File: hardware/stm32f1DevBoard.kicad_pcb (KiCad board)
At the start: 2 copper layers, 105.4 x 62.2 mm, 67 parts, among them J1 USB_2, J2 POWER_JACK, J3 SDCARD, M1 Mounting Hole, M2 Mounting Hole, M3 Mounting Hole, M4 Mounting Hole, P1 JTAG, P2 P20, P3 P20, P4 WIFIDEBUG, Q1 MOSFET-P, U1 STM32F102C6, U2 MRF24WB0MX, U3 LM358, U4 VREG-X-5, U5 VREG-5-3.3, X1 32,768Hz, X2 20MHz

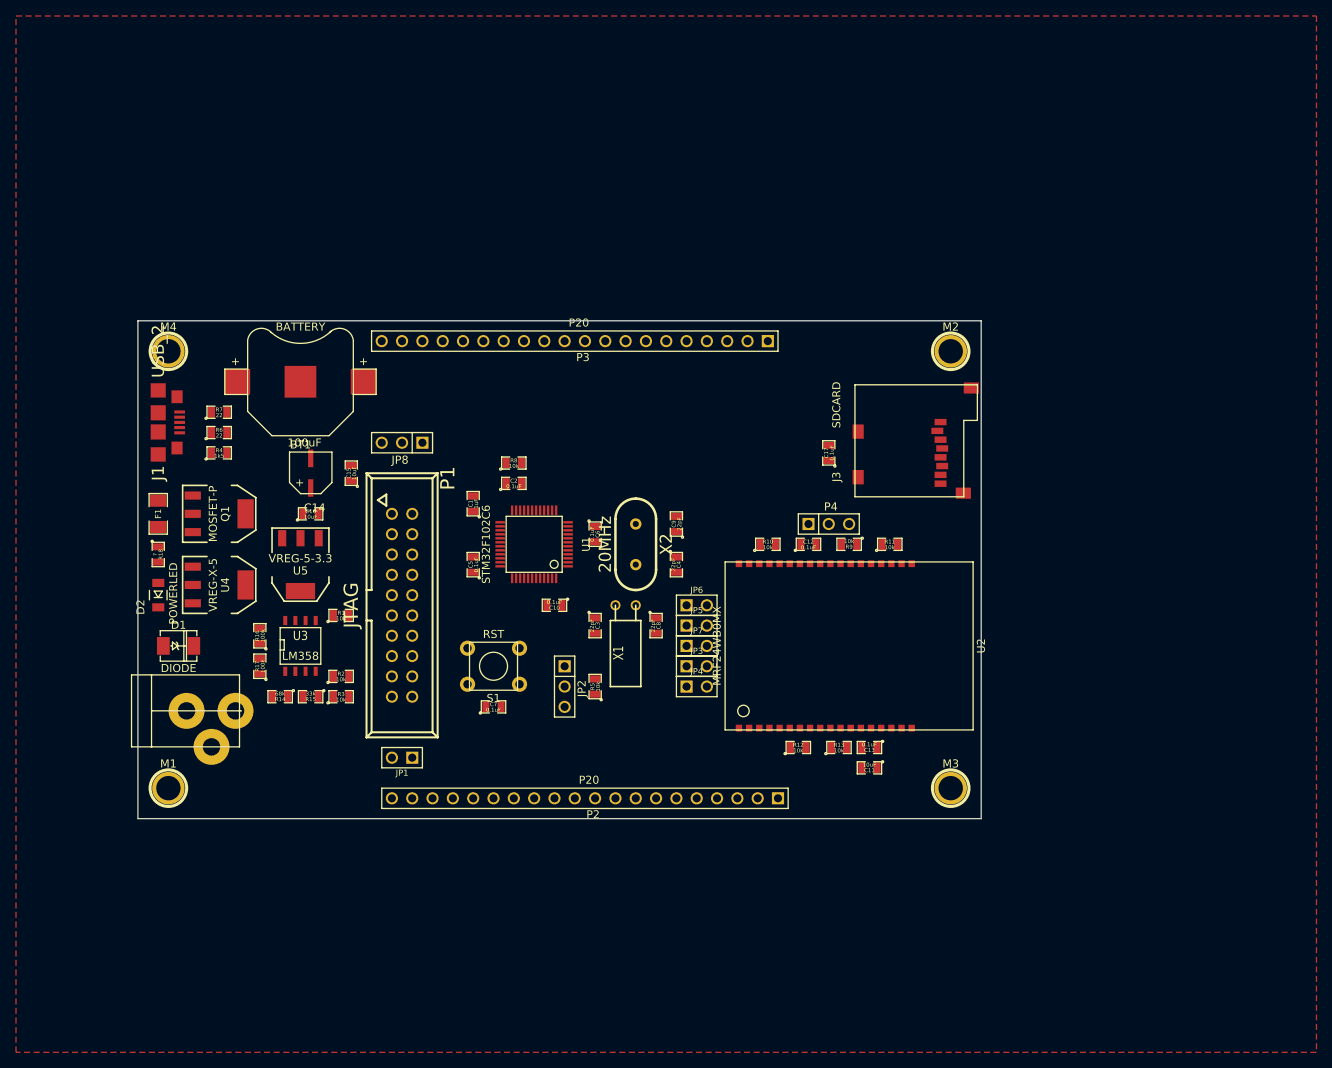
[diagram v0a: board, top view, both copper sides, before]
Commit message: layout complete
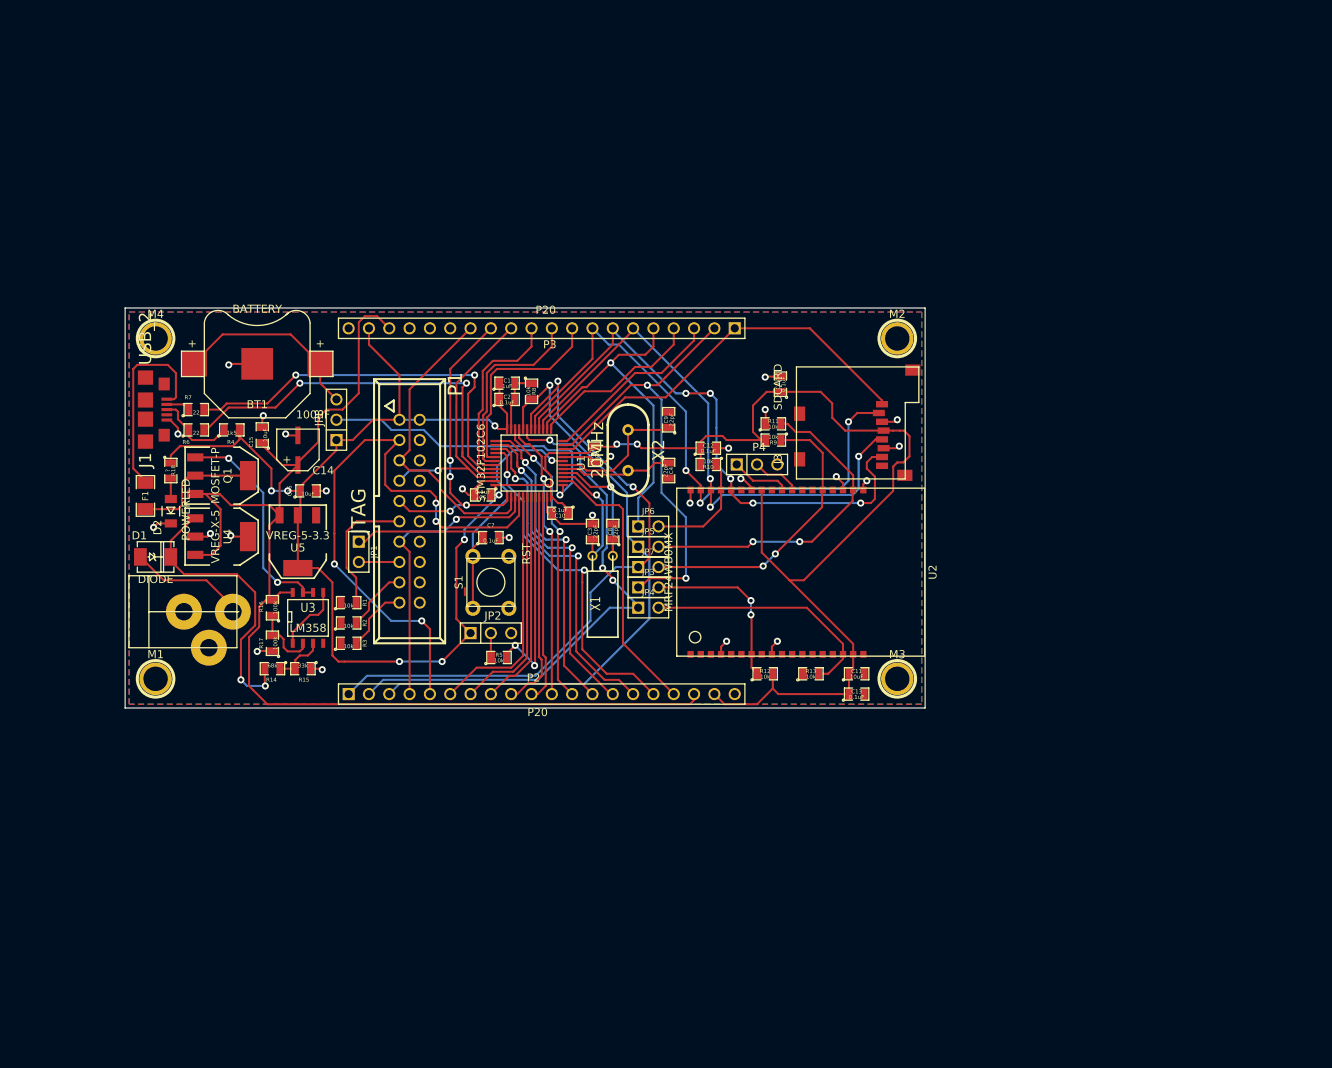
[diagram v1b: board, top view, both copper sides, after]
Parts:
- moved JP1 26.3 mm to (129.2, 130.5), turned to 270 degrees
- moved C7 21.2 mm to (145.7, 128.7)
- moved R11 20.9 mm to (181.0, 114.5)
- moved C12 17.4 mm to (172.9, 117.5)
- moved R9 16.1 mm to (181.0, 116.5)
- moved C1 15.6 mm to (147.8, 109.4), turned to 0 degrees
- moved P2 15.3 mm to (150.8, 148.3), turned to 0 degrees
- moved M3 15.2 mm to (196.5, 146.4)
- moved M1 13.8 mm to (103.8, 146.4)
- moved C9 13.1 mm to (167.9, 114.0)
- moved C8 12.9 mm to (161.0, 127.9), turned to 90 degrees
- moved R5 12.6 mm to (146.7, 143.7), turned to 0 degrees
- moved R10 12.5 mm to (172.9, 119.6), turned to 180 degrees
- moved J2 12.4 mm to (110.2, 137.5)
- moved C15 12.1 mm to (117.1, 115.9)
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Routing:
- net +3.3V: track 0.00 -> 294.5 mm, vias 0 -> 9
- net +5V: track 0.00 -> 146.7 mm
- net nWIFICS: track 0.00 -> 81.2 mm, vias 0 -> 2
- net WIFIHIBERNATE: track 0.00 -> 78.0 mm, vias 0 -> 1
- net MOSI: track 0.00 -> 75.1 mm, vias 0 -> 3
- net nJTRST: track 0.00 -> 74.8 mm, vias 0 -> 4
- net GND: track 0.00 -> 72.5 mm, vias 0 -> 25
- net MISO: track 0.00 -> 71.6 mm, vias 0 -> 5
- net SCK: track 0.00 -> 71.0 mm, vias 0 -> 3
- net nWIFIWP: track 0.00 -> 69.7 mm, vias 0 -> 3
- net nWIFIRESET: track 0.00 -> 57.6 mm, vias 0 -> 2
- net SDCS: track 0.00 -> 50.3 mm
- net N-0000016: track 0.00 -> 50.1 mm, vias 0 -> 2
- net N-0000017: track 0.00 -> 49.5 mm, vias 0 -> 2
- net nRST: track 0.00 -> 49.0 mm, vias 0 -> 1
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- added copper zone on B.Cu, net GND
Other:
- board size 105.4 x 62.2 mm -> 100 x 50 mm
- net class Default: clearance 0.254 -> 0.2032
- rule trace_clearance: 0.254 -> 0.2032
